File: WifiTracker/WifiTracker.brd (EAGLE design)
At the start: 161.3 x 81 mm, 29 parts, among them IC1 TS1117CP33-R0, Q1 BSS123, Q2 BSS123, Y1 16MHz

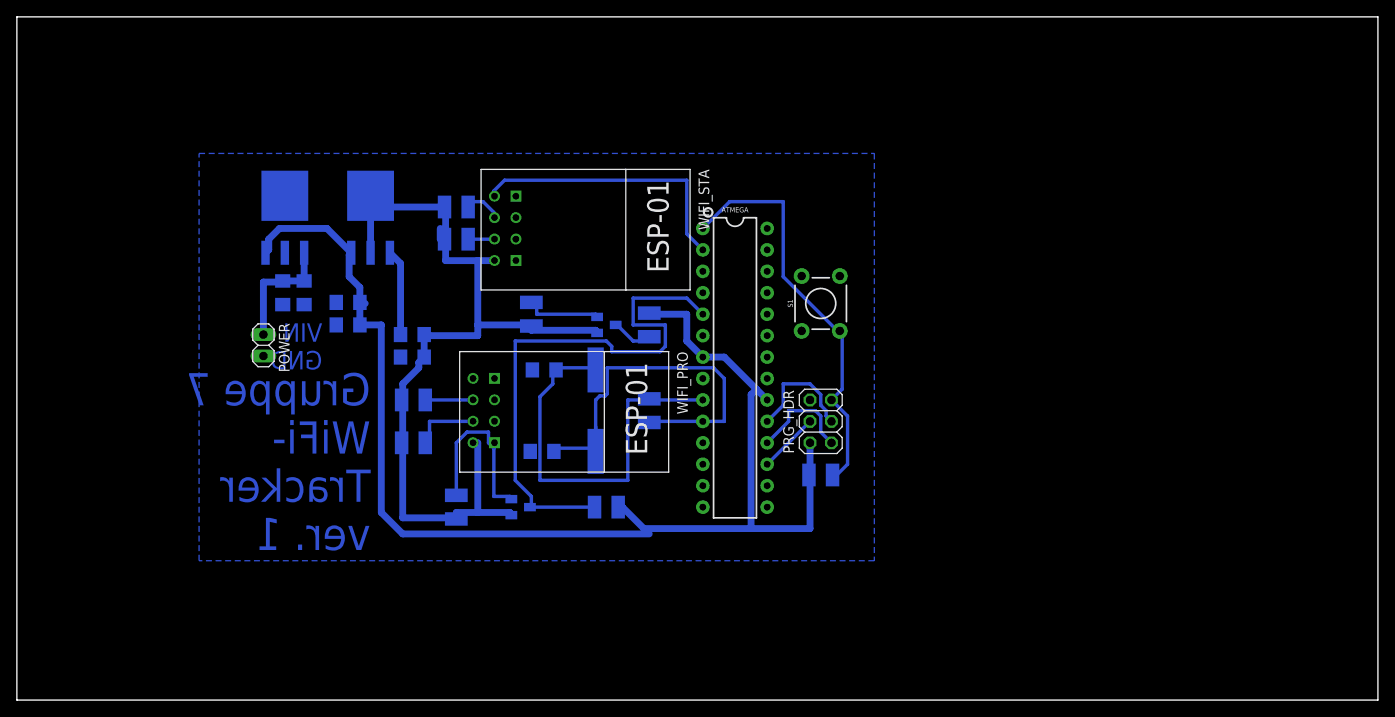
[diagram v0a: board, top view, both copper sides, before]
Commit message: Prepare to print
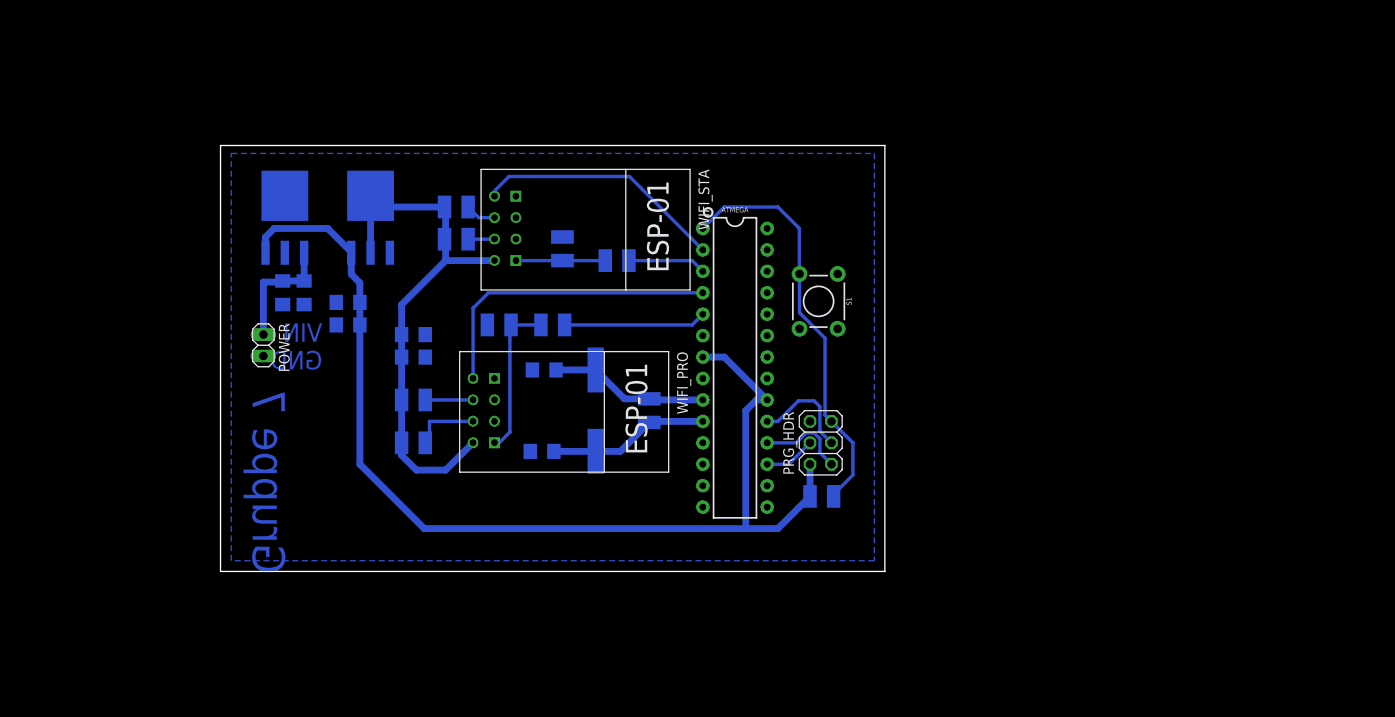
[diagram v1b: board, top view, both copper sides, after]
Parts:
- removed Q1, Q2: BSS123, transistor-small-signal:SOT23
- R10, R8: value 10kΩ -> 2.2kΩ
- R7, R9: value 10kΩ -> 1kΩ
- moved R8 25.0 mm to (57.1, 44.5)
- moved R7 24.4 mm to (63.5, 44.5), turned to 0 degrees
- moved R10 13.7 mm to (64.6, 53.5), turned to 90 degrees
- moved R9 12.0 mm to (71.1, 52.1), turned to 0 degrees
- moved R6 2.54 mm to (95.4, 24.1)
- moved PRG_HDR 2.54 mm to (95.2, 30.5)
- moved S1 0.36 mm to (95.0, 47.2), turned to 270 degrees
- moved C6 0.13 mm to (47.0, 40.6), turned to 180 degrees
- moved C9 0.13 mm to (47.0, 43.3), turned to 180 degrees
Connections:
- removed net N$1: WIFI_PRO.TX
- removed net N$2: WIFI_STA.RX
- removed net N$3: Q1.2, R7.2, WIFI_PRO.RX
- removed net N$4: Q2.2, R9.2
- removed net PRO_RXD1: Q2.3, R10.2
- new net AT_STXD: ATMEGA.5, R7.1
- new net AT_TXD: ATMEGA.3, R9.1
- net 3VCC: no longer Q1.1, Q2.1, R7.1, R9.1
- net 5VCC: no longer R10.1, R8.1
- net GND: now also R10.2, R8.2
- net PRO_RXD: now also R7.2, R8.1, WIFI_PRO.RX; no longer ATMEGA.5, Q1.3, R8.2
- net PRO_TXD: now also WIFI_PRO.TX
- net STA_RXD: now also R10.1, R9.2, WIFI_STA.RX; no longer ATMEGA.3
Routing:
- net PRO_RXD: track 65.8 -> 18.7 mm
- net 3VCC: track 106.8 -> 64.2 mm
- net PRO_TXD: track 0.00 -> 36.3 mm
- net XTAL1: track 48.0 -> 18.9 mm
- net XTAL2: track 47.7 -> 19.1 mm
- net 5VCC: track 151.8 -> 127.9 mm
- net N$3: track 22.1 -> 0.00 mm
- net AT_STXD: track 0.00 -> 16.9 mm
- net STA_RXD: track 0.00 -> 10.6 mm
- net GND: track 10.2 -> 0.00 mm
- net N$4: track 10.0 -> 0.00 mm
- net AT_TXD: track 0.00 -> 9.29 mm
- net PRO_RXD1: track 5.27 -> 0.00 mm
- net STA_TXD: track 33.1 -> 29.6 mm
- net MISO: track 12.6 -> 10.6 mm
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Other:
- board size 161.3 x 81 mm -> 78.7 x 50.5 mm
- board text added: "Gruppe 7"
- board text removed: "Gruppe 7 WiFi- Tracker ver. 1"
